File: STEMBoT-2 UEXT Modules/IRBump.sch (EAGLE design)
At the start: 23 parts, among them IC1 LMV324DR2G, IC2 LMV324DR2G, IC3 74HC165PW,118, Q1 MMBT3904LP-7, U1 SN74HC148D

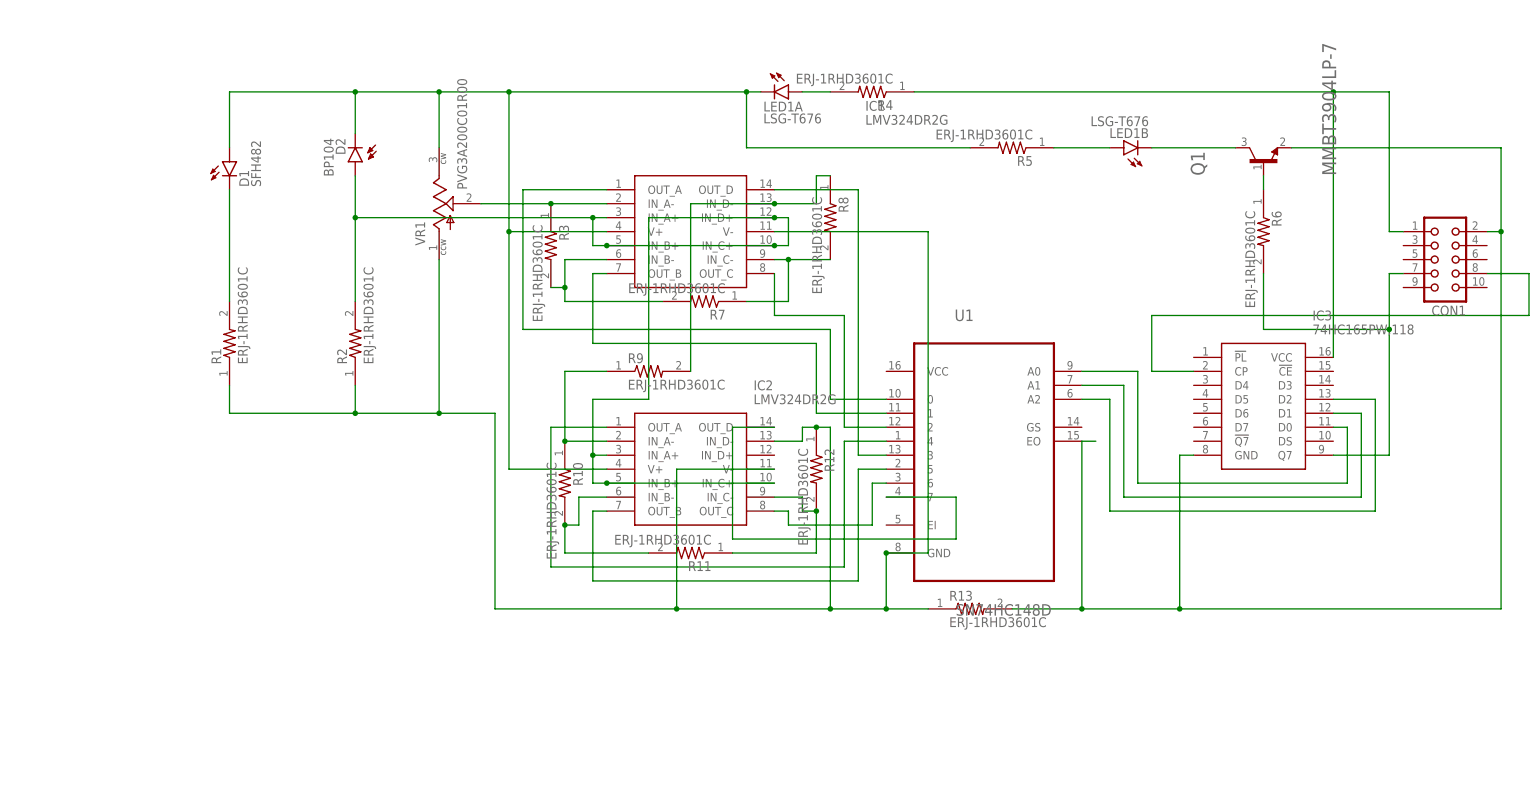
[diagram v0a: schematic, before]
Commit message: Once again, updating ADC shematics and boards. Used autorouter.
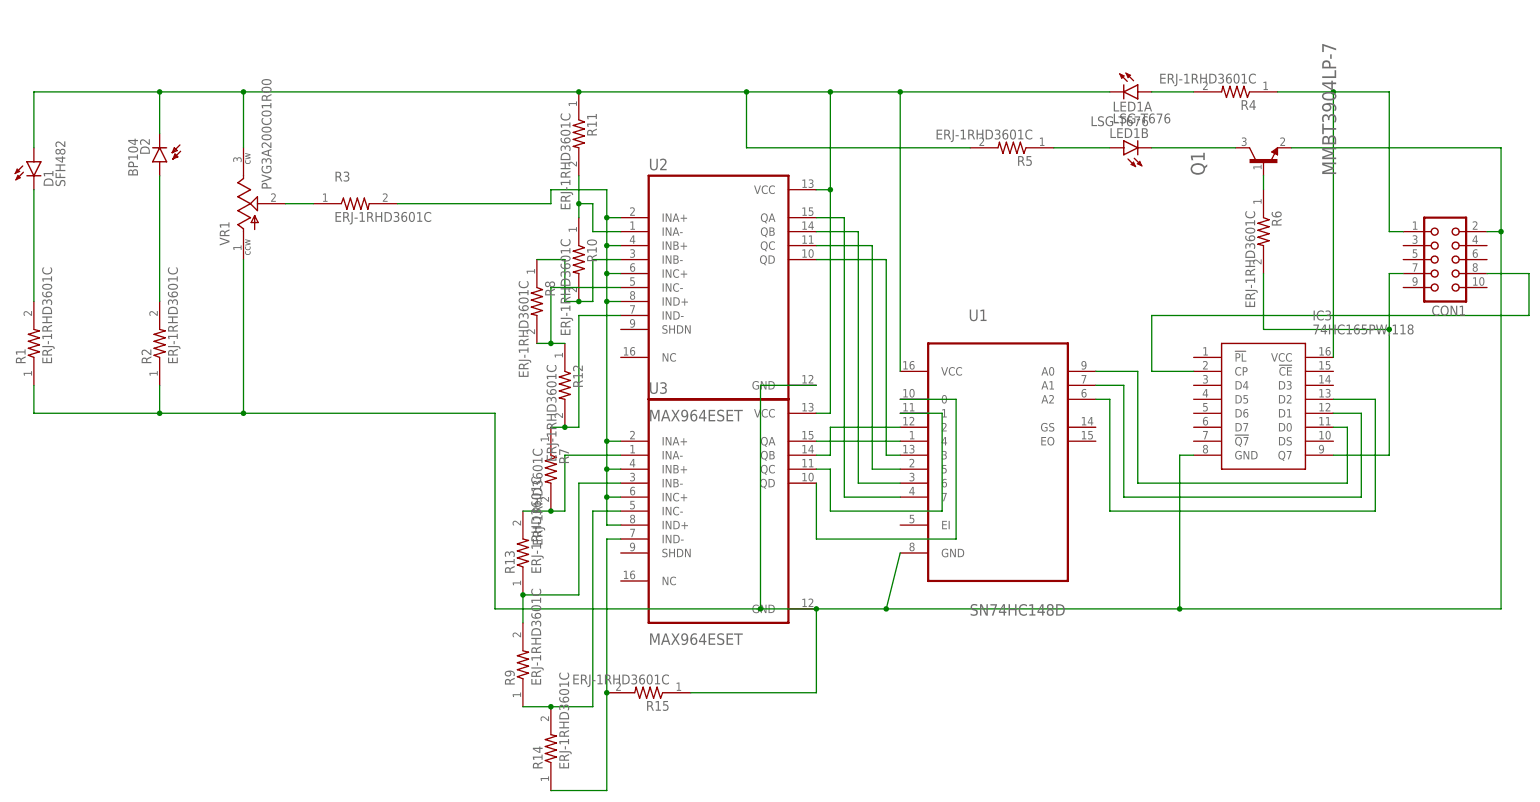
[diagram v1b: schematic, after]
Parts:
- removed IC1, IC2: LMV324DR2G, LMV324DR2G:LMV324DR2G
- added R14, R15: ERJ-1RHD3601C, Resistor:ERJ-1RHD3601C
- added U2, U3: MAX964ESET, MAX964ESET:MAX964ESET
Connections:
- removed net N$21: IC1.V-, IC2.IN_D-, IC2.V-, R1.1, R12.1, R13.1, R2.1, U1.GND, VR1.CCW
- new net N$27: U1.2, U3.QB
- new net N$32: U1.1, U3.QC
- new net N$33: U1.0, U3.QD
- net N$1: now also R3.2, U2.INA+, U2.INB+, U2.INC+, U2.IND+, U3.INA+, U3.INB+, U3.INC+, U3.IND+; no longer IC2.OUT_C, U1.6
- net N$11: now also R10.2, R8.1, U2.INB-; no longer IC2.OUT_A, U1.4
- net N$13: now also R12.1, R8.2, U2.INC-; no longer IC2.OUT_B, U1.5
- net N$14: no longer IC1.IN_A-
- net N$15: now also R12.2, R7.1, U2.IND-; no longer IC1.IN_B-, R3.2, R7.2
- net N$16: now also R13.2, R7.2, U3.INA-; no longer IC1.IN_C-, R7.1, R8.2
- net N$18: now also R13.1, U3.INB-; no longer IC1.IN_D-, R8.1
- net N$19: now also R14.2, U3.INC-; no longer IC2.IN_A-, R10.1
- net N$20: now also R14.1, R15.2, U3.IND-; no longer IC2.IN_B-, R10.2, R11.2
- net N$22: now also U1.6, U2.QB; no longer IC1.OUT_D, U1.3
- net N$23: now also U1.5, U2.QC; no longer IC1.OUT_C, U1.2
- net N$24: now also U1.3, U2.QD; no longer IC1.OUT_B, U1.1
- net N$25: now also U1.4, U3.QA; no longer IC1.OUT_A, U1.0
- net N$4: now also R1.1, R15.1, R2.1, U1.GND, U2.GND, U3.GND, VR1.CCW; no longer R13.2, U1.EO
- net N$5: now also U1.7, U2.QA; no longer IC2.IN_C-, R11.1, R12.2
- net N$6: now also R11.1, U1.VCC, U2.VCC, U3.VCC; no longer IC1.V+, IC2.V+
- net N$7: no longer IC1.IN_A+, IC1.IN_B+, IC1.IN_C+, IC1.IN_D+, IC2.IN_A+, IC2.IN_B+, IC2.IN_C+
- net N$9: now also R10.1, R11.2, U2.INA-; no longer IC2.OUT_D, U1.7
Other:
- moved on the sheet: D1, D2, LED1A, R1, R10, R11, R12, R13, R2, R3, R4, R7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
